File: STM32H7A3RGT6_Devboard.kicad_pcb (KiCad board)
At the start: 2 copper layers, 63.8 x 25.7 mm, 34 parts, among them J1 USB_C_Receptacle_USB2.0_14P, J2 Conn_01x04_Socket, J3 Conn_01x25_PinHeader, J4 Conn_01x25_PinHeader, SW1 RESET, SW2 BOOT, U1 STM32H7A3RGT6, U2 AP2127N-3.3TRG1, U3 USBLC6-2SC6, Y1 12MHz

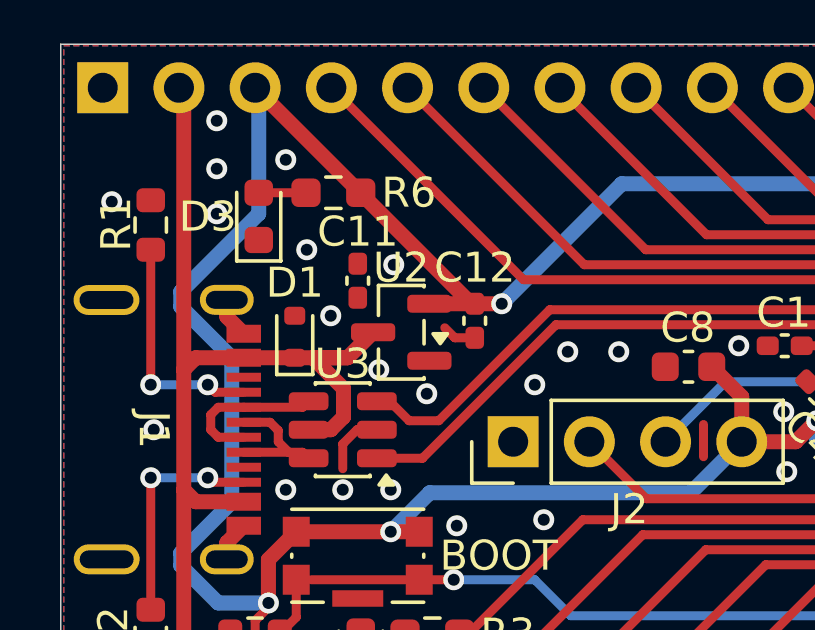
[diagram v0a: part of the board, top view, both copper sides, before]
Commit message: Fix more DRC check errors
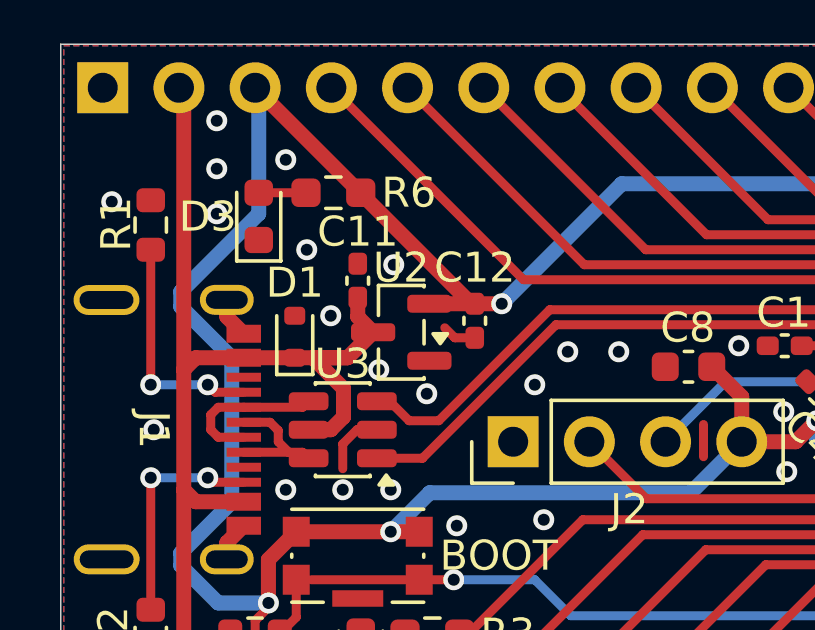
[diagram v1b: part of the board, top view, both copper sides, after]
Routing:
- net VBUS: track 36.8 -> 38.2 mm
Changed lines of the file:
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@@
 		(capping no)
 		(filling no)
-		(zone_defaults)
 		(pcbplotparams
 			(layerselection 0x00000000_00000000_55555555_5755f5ff)
@@
 	)
 	(segment
+		(start 106.8 95.6)
+		(end 106.8 96.2375)
+		(width 0.5)
+		(layer "F.Cu")
+		(net "VBUS")
+	)
+	(segment
 		(start 105.3 97.6)
 		(end 106.325 98.625)
@@
 		(width 0.5)
 		(layer "F.Cu")
+		(net "VBUS")
+	)
+	(segment
+		(start 106.8 96.2375)
+		(end 107.3125 96.75)
+		(width 0.5)
+		(layer "F.Cu")
